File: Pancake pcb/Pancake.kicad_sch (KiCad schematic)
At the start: 85 parts, among them U1 Frood

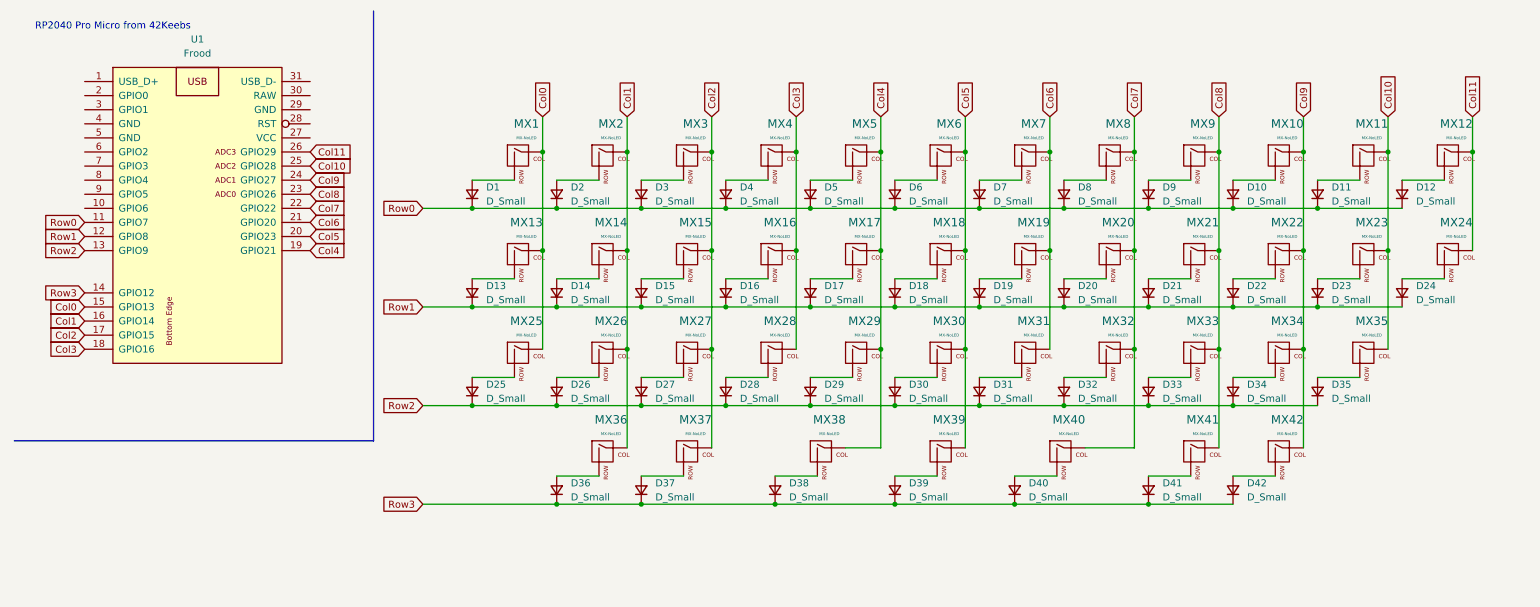
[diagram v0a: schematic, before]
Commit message: A lot of modification
addition of a jst cable and other
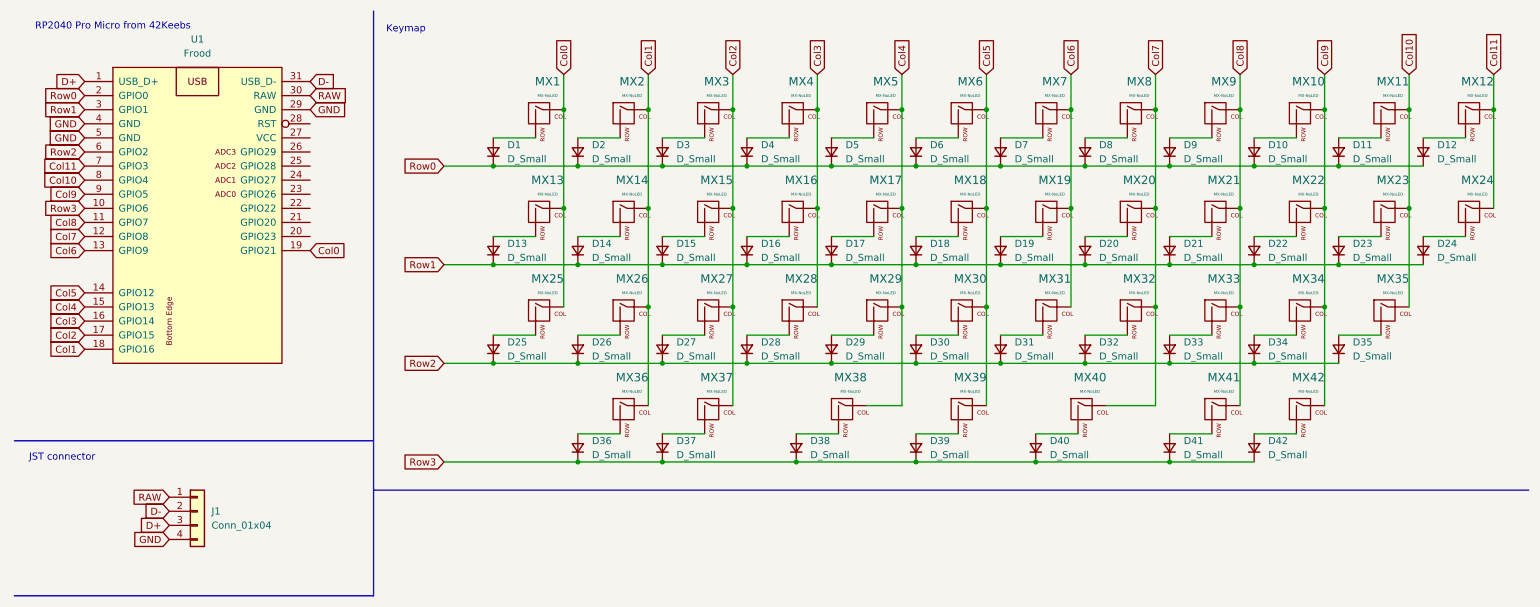
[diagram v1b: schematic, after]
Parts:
- added J1: Conn_01x04, Connector_JST:JST_SH_BM04B-SRSS-TB_1x04-1MP_P1.00mm_Vertical, symbol PCM_4ms_Connector:Conn_01x04
- D1, D10, D11, D12, D13, D14, D15, D16, D17, D18, D19, D2, D20, D21, D22, D23, D24, D25, D26, D27, D28, D29, D3, D30, D31, D32, D33, D34, D35, D36, D37, D38, D39, D4, D40, D41, D42, D5, D6, D7, D8, D9: footprint (none) -> Diode_SMD:D_SOD-123
- MX1, MX10, MX11, MX14, MX15, MX16, MX17, MX18, MX19, MX2, MX20, MX21, MX22, MX23, MX24, MX26, MX27, MX28, MX29, MX3, MX30, MX31, MX32, MX33, MX34, MX37, MX39, MX4, MX41, MX5, MX6, MX7, MX8, MX9: footprint (none) -> ScottoKeebs_MX:MX_PCB_1.00u
- MX12, MX13, MX35, MX36, MX42: footprint (none) -> ScottoKeebs_MX:MX_PCB_1.25u
- MX25: footprint (none) -> ScottoKeebs_MX:MX_PCB_1.50u
- MX38, MX40: footprint (none) -> ScottoKeebs_MX:MX_PCB_2.00u
- U1: footprint 42keebs:Frood_PinHeader_2x13+5_P2.54mm_Labels_Top -> footprints:Frood_PinHeader_2x13+5_P2.54mm_Labels_Top
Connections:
- net Col0: now also U1.19 (GPIO21); no longer U1.15 (GPIO13)
- net Col1: now also U1.18 (GPIO16); no longer U1.16 (GPIO14)
- net Col10: now also U1.8 (GPIO4); no longer U1.25 (GPIO28)
- net Col11: now also U1.7 (GPIO3); no longer U1.26 (GPIO29)
- net Col3: now also U1.16 (GPIO14); no longer U1.18 (GPIO16)
- net Col4: now also U1.15 (GPIO13); no longer U1.19 (GPIO21)
- net Col5: now also U1.14 (GPIO12); no longer U1.20 (GPIO23)
- net Col6: now also U1.13 (GPIO9); no longer U1.21 (GPIO20)
- net Col7: now also U1.12 (GPIO8); no longer U1.22 (GPIO22)
- net Col8: now also U1.11 (GPIO7); no longer U1.23 (GPIO26)
- net Col9: now also U1.9 (GPIO5); no longer U1.24 (GPIO27)
- net Row0: now also U1.2 (GPIO0); no longer U1.11 (GPIO7)
- net Row1: now also U1.3 (GPIO1); no longer U1.12 (GPIO8)
- net Row2: now also U1.6 (GPIO2); no longer U1.13 (GPIO9)
- net Row3: now also U1.10 (GPIO6); no longer U1.14 (GPIO12)
- net D+: now reaches U1.1 (USB_D+)
- net D+: now also J1.3 (Pin_3)
- net GND: now reaches U1.29 (GND)
- net GND: now also U1.4 (GND), U1.5 (GND), J1.4 (Pin_4)
- net RAW: now reaches U1.30 (RAW)
- net RAW: now also J1.1 (Pin_1)
- net D-: now reaches U1.31 (USB_D-)
- net D-: now also J1.2 (Pin_2)
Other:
- note added: "JST connector"
- note added: "Keymap"
- moved on the sheet: D1, D10, D11, D12, D13, D14, D15, D16, D17, D18, D19, D2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
